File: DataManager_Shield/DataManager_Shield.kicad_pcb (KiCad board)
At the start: 4 copper layers, 78 x 70 mm, 79 parts, among them J1 CAR_IN, J2 aux_pin, J3 CAR_OUT, J4 Mode_Selector, K1 IM03, K2 IM03, Q10 AO3400A, Q9 AO3400A, U1 TLP291-4, U2 MCP4725xxx-xCH, U3 TLP291-4, U4 PCA9306

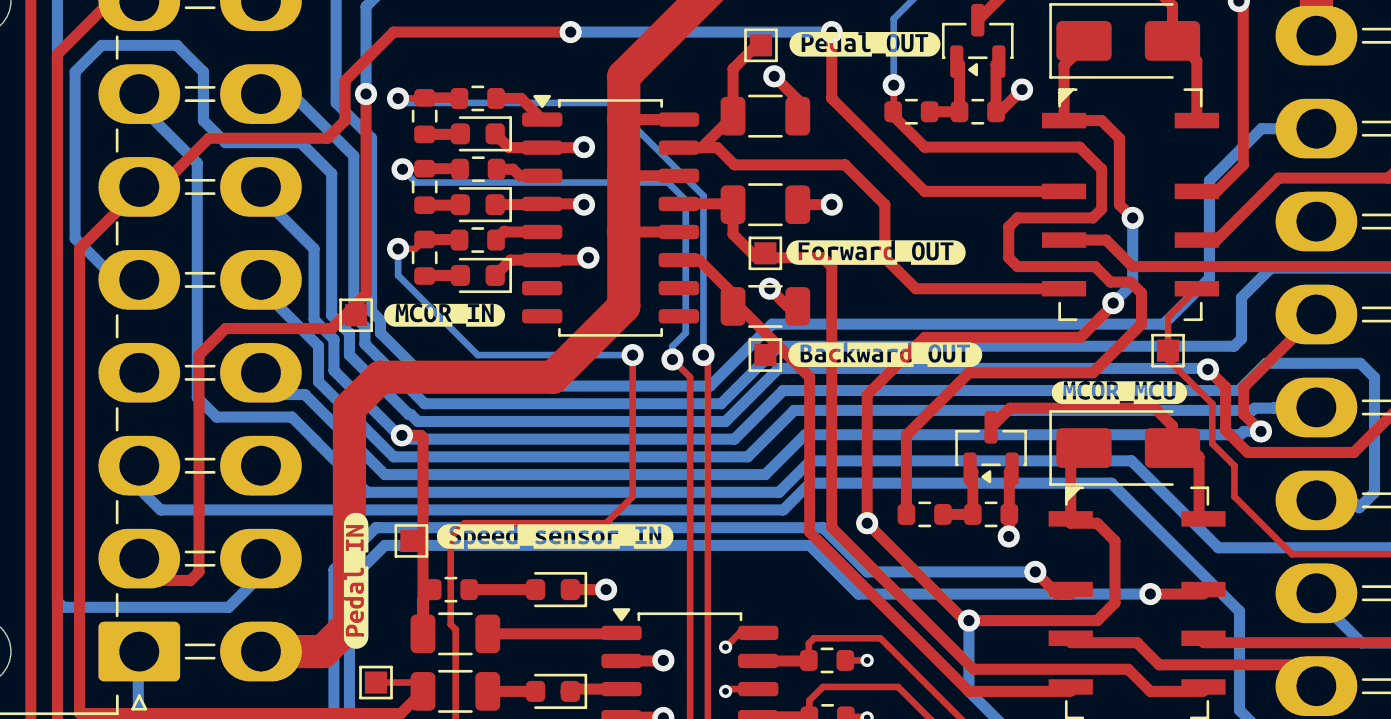
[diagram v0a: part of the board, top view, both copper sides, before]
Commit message: up
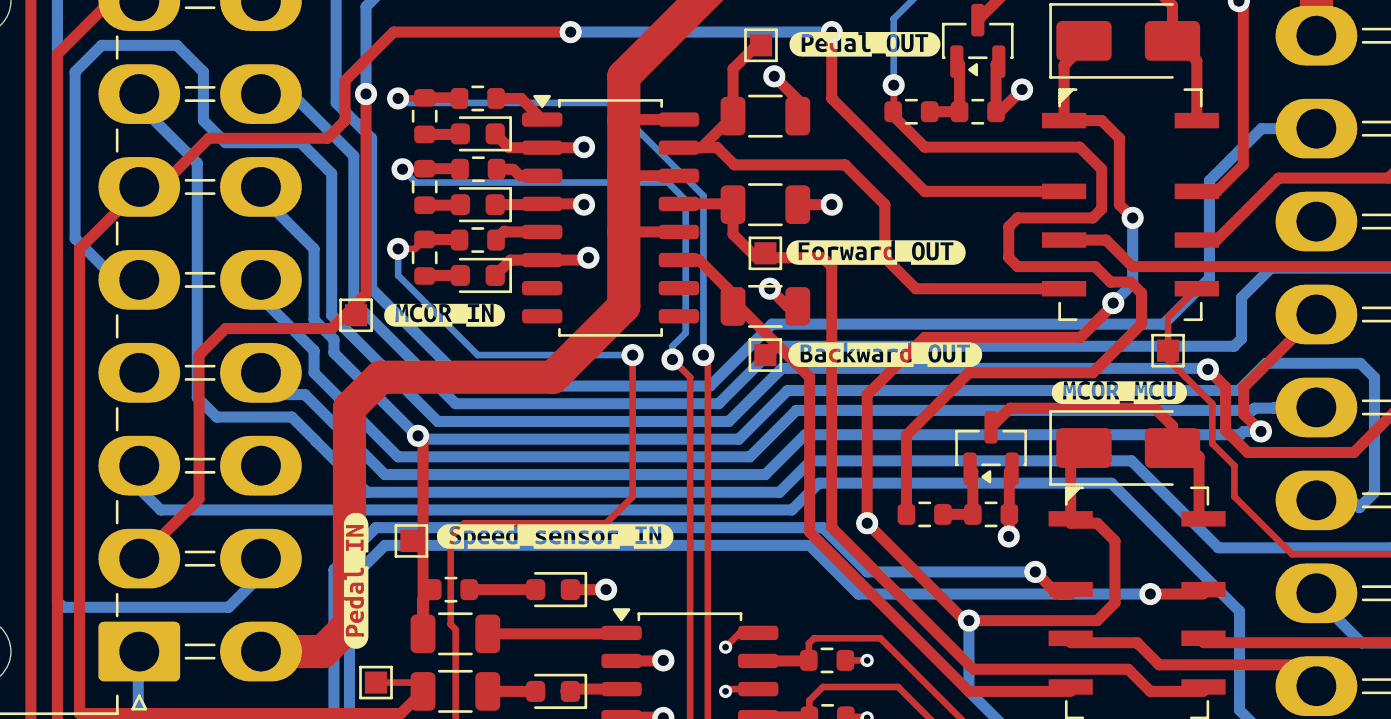
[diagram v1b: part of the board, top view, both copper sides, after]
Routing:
- net /Relays/MCOR_Speed_Control_IN: track 155.9 -> 154.5 mm
- net /Relays/Speed_Sensor: track 79.4 -> 78.2 mm
- net /Relays/Key_Switch_In: track 118.7 -> 117.7 mm
- net /Relays/ Speed_Sensor_Supply_Out / about_15V: track 97.1 -> 96.3 mm
- net /Relays/Power_Down/Charger_Interlock: track 90.9 -> 90.3 mm
